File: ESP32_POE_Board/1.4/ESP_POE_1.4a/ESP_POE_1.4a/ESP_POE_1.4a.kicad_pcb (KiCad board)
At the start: 4 copper layers, 40 x 40 mm, 67 parts, among them J2 SI-46020-F, J3 HMTSW-102-X-X-S-X, J4 20021111-00012T4LF, J6 20021111-00012T4LF, T1 LMUN2211LT1G(SOT-23), U2 TPS2376PW(TSSOP-8), U4 LAN8710A-EZC(QFN32), U5 TX4138(ESOIC-8)

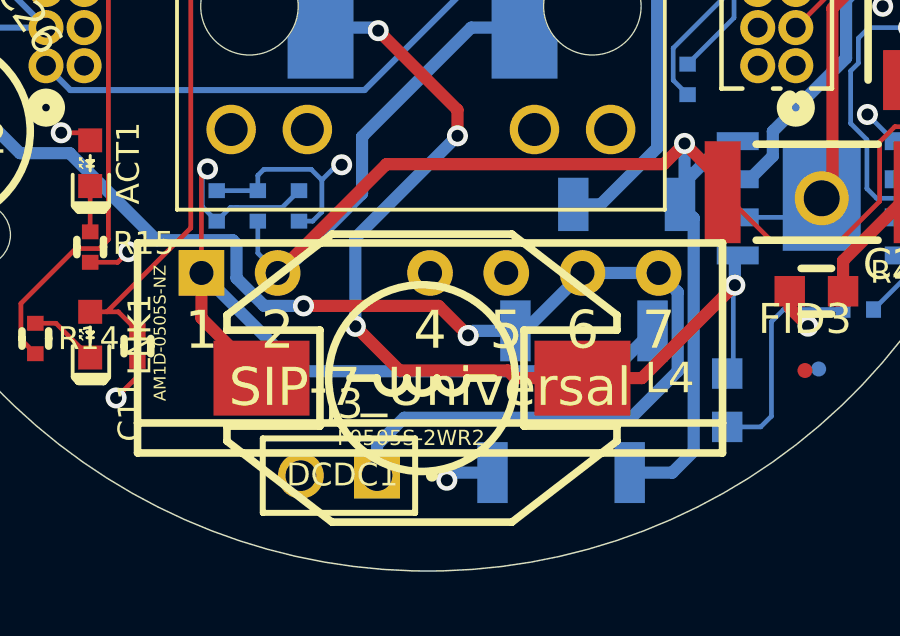
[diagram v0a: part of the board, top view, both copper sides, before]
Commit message: 1.4a half bom
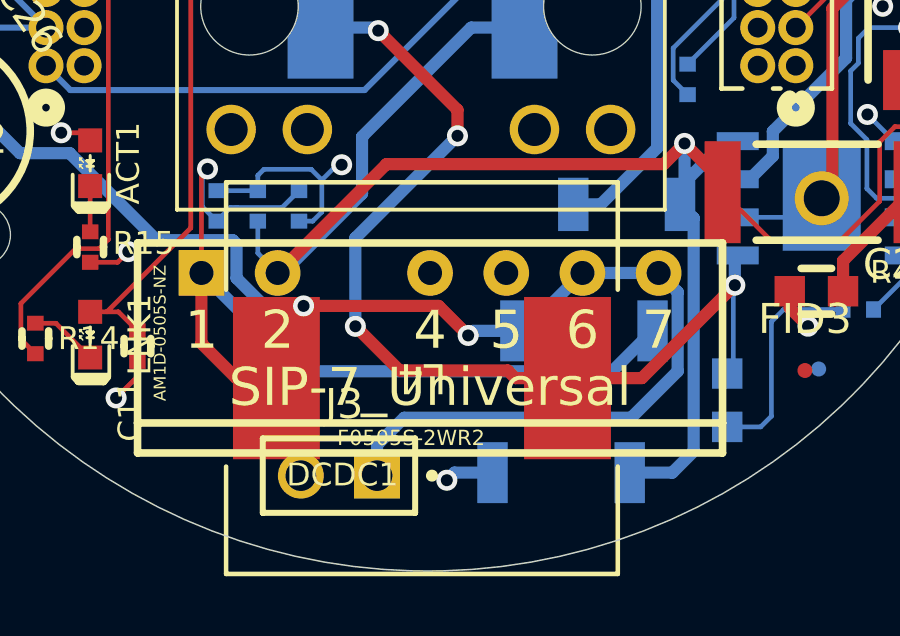
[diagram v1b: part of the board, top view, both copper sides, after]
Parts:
- C20: value NA(1.0nF/3kV/10%/X7R/SMD/1808(VISHAY-VJ1808Y102KBHAT4X_Farnell-2407291)) -> 1.0nF/3kV/10%/X7R/SMD/1808(VISHAY-VJ1808Y102KBHAT4X_Farnell-2407291)
- L4: footprint OLIMEX_RLC-FP:DBS135 -> SRR1240-330M:IND_BOURNS_SRR1240
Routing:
- net /5V_DCDC: track 40.7 -> 41.7 mm
